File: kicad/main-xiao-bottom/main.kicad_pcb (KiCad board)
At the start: 2 copper layers, 41 x 41.5 mm, 22 parts, among them J1 Conn_01x14, J10 Conn_01x01_Pin, J11 Conn_01x01_Pin, J12 Conn_01x01_Pin, J13 Conn_01x01_Pin, J14 Conn_01x05_Socket, J2 Conn_01x14_Socket, J3 Conn_01x01_Pin, J4 Conn_01x03_Socket, J5 Conn_01x06, J6 Conn_01x08, J7 Conn_01x01_Pin, J8 Conn_01x01_Pin, J9 Conn_01x01_Pin

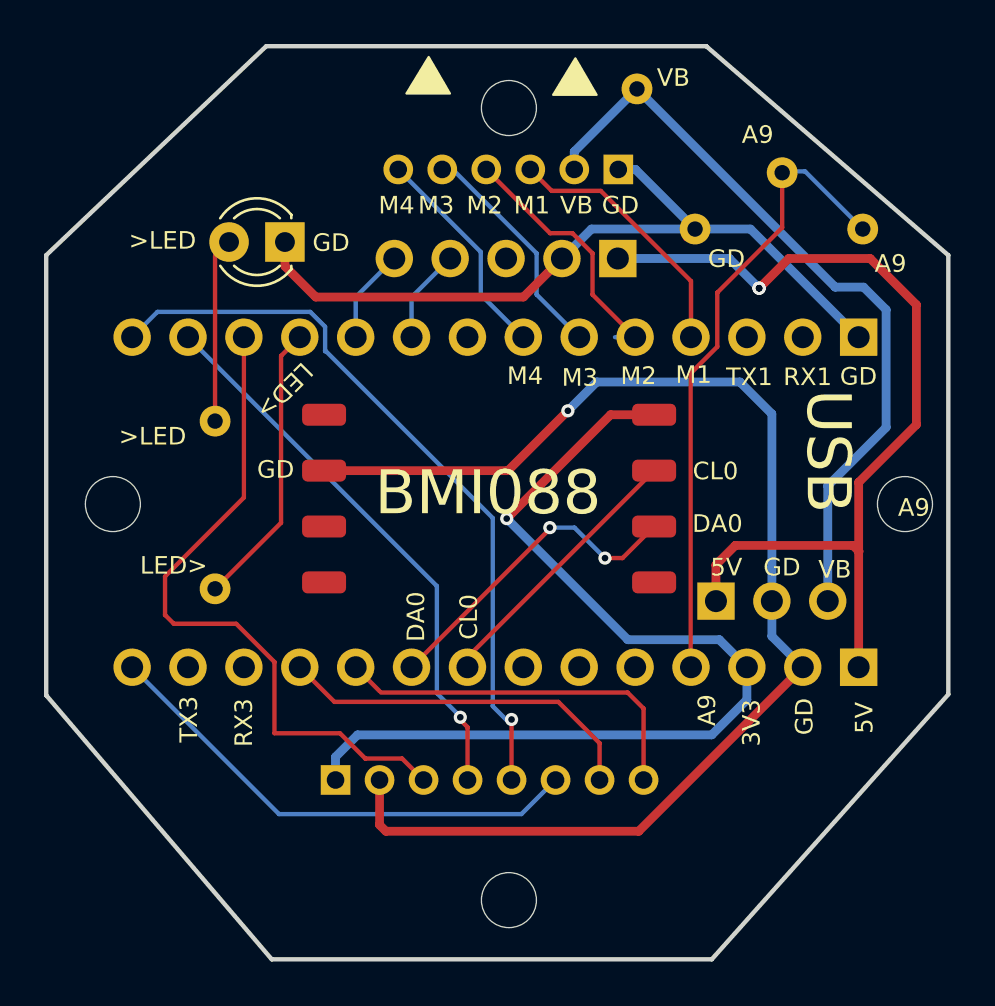
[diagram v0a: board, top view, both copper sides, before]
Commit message: modified:   kicad/main-xiao-bottom/main.kicad_pcb
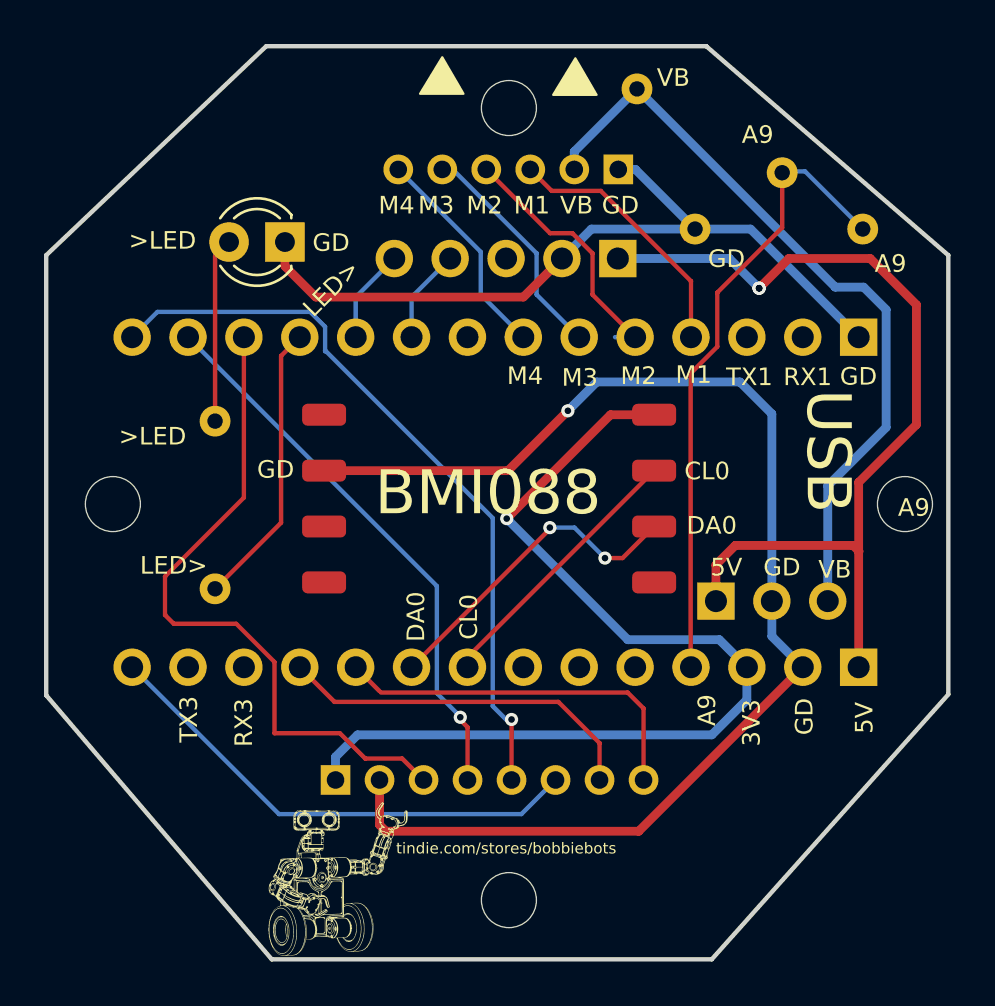
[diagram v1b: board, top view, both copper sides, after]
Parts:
- added G***: LOGO, LOGO, F.Cu at (138.1, 102.3)
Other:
- board text added: "tindie.com/stores/bobbiebots"
